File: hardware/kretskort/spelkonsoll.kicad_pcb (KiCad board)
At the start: 2 copper layers, 2 parts, among them U2 ESP32-DEVKITC-32D, U3 ILI9488

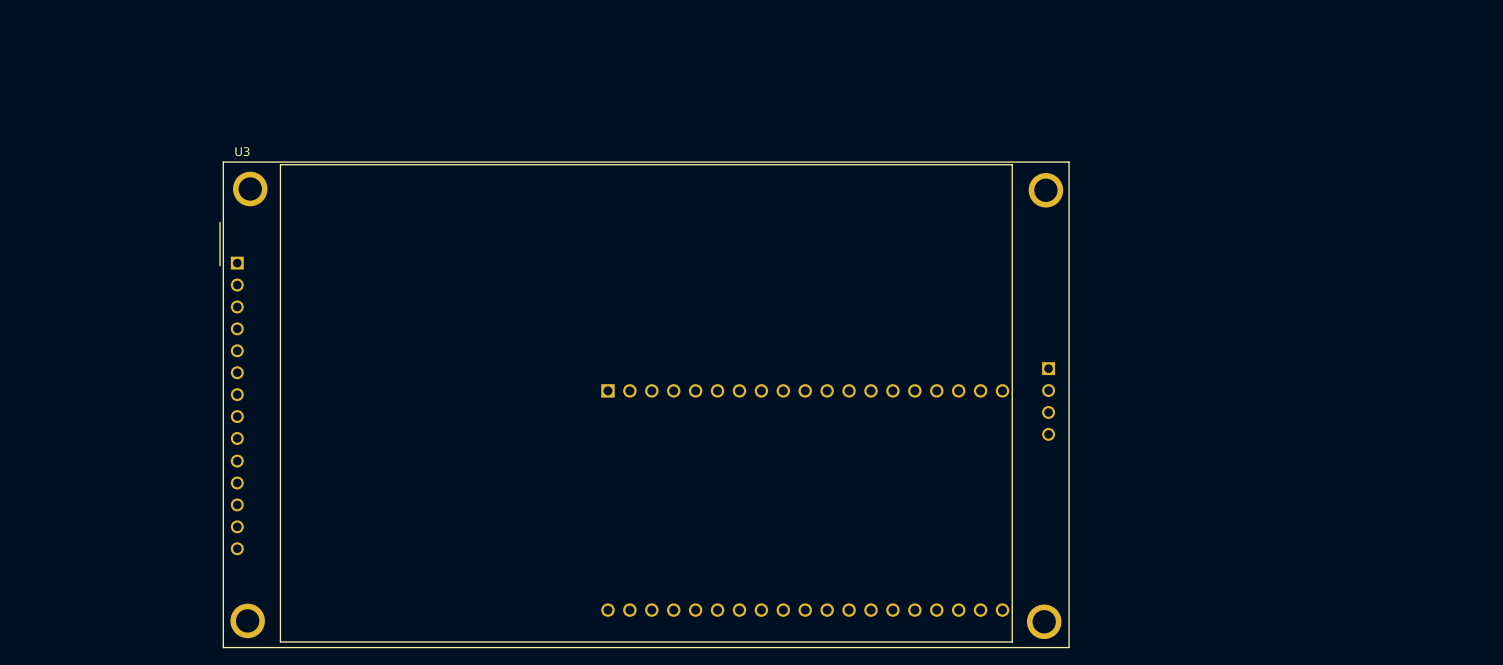
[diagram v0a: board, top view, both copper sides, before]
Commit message: more circuit board kicad files
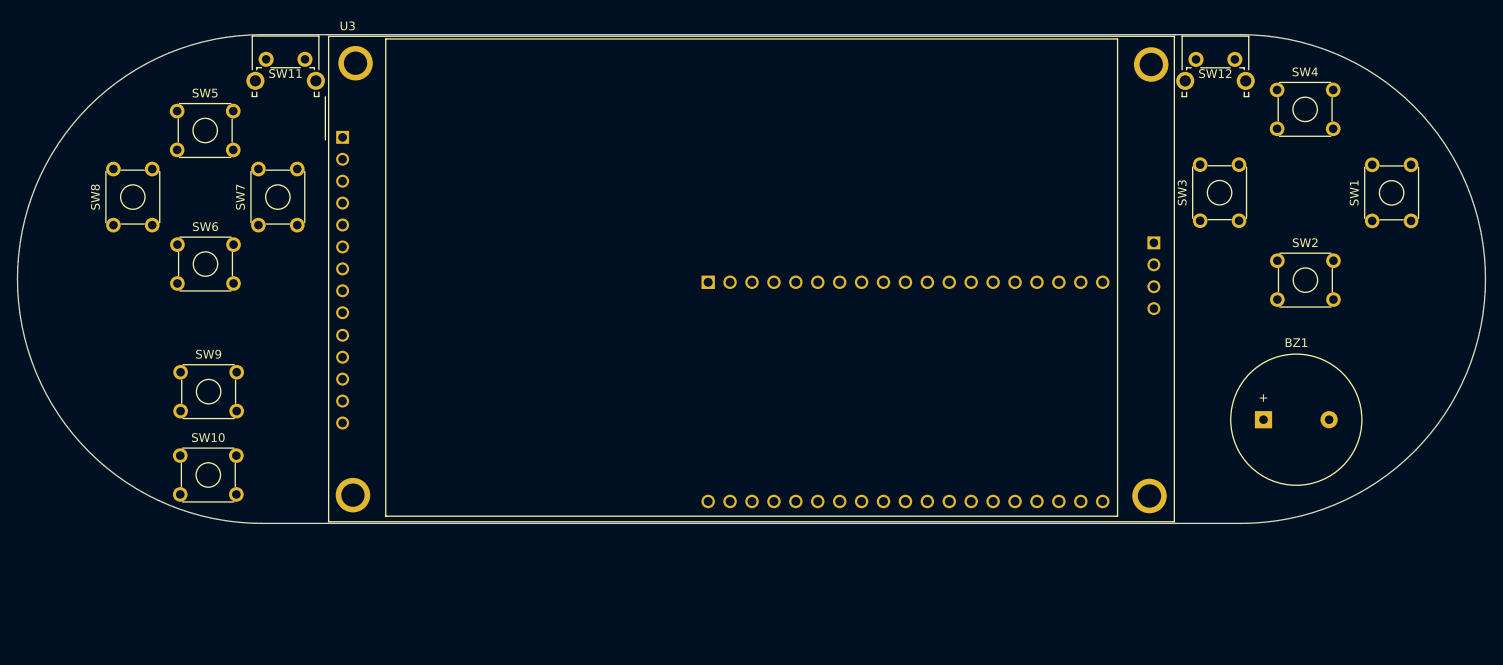
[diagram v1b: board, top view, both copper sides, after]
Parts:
- added BZ1: Buzzer, Buzzer_Beeper:Buzzer_15x7.5RM7.6, F.Cu at (204.8, 113.8)
- added SW1: SW_Push, Button_Switch_THT:SW_TH_Tactile_Omron_B3F-10xx, F.Cu at (217.4, 90.8)
- added SW10: SW_Push, Button_Switch_THT:SW_TH_Tactile_Omron_B3F-10xx, F.Cu at (79.3, 118.0)
- added SW11: SW_Push, Button_Switch_THT:SW_Tactile_SPST_Angled_PTS645Vx83-2LFS, F.Cu at (89.2, 72.1)
- added SW12: SW_Push, Button_Switch_THT:SW_Tactile_SPST_Angled_PTS645Vx83-2LFS, F.Cu at (197.0, 72.1)
- added SW2: SW_Push, Button_Switch_THT:SW_TH_Tactile_Omron_B3F-10xx, F.Cu at (206.4, 95.4)
- added SW3: SW_Push, Button_Switch_THT:SW_TH_Tactile_Omron_B3F-10xx, F.Cu at (197.5, 90.8)
- added SW4: SW_Push, Button_Switch_THT:SW_TH_Tactile_Omron_B3F-10xx, F.Cu at (206.4, 75.6)
- added SW5: SW_Push, Button_Switch_THT:SW_TH_Tactile_Omron_B3F-10xx, F.Cu at (78.9, 78.1)
- added SW6: SW_Push, Button_Switch_THT:SW_TH_Tactile_Omron_B3F-10xx, F.Cu at (78.9, 93.5)
- added SW7: SW_Push, Button_Switch_THT:SW_TH_Tactile_Omron_B3F-10xx, F.Cu at (88.3, 91.3)
- added SW8: SW_Push, Button_Switch_THT:SW_TH_Tactile_Omron_B3F-10xx, F.Cu at (71.5, 91.3)
- added SW9: SW_Push, Button_Switch_THT:SW_TH_Tactile_Omron_B3F-10xx, F.Cu at (79.3, 108.3)
- moved U3 19.0 mm to (150.2, 106.6)
- moved U2 17.1 mm to (160.2, 110.6)
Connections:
- U2 pad 10: Net-(U2-Pad10) -> BTN_SELECT
- U2 pad 11: Net-(U2-Pad11) -> BTN_DP_UP
- U2 pad 12: Net-(U2-Pad12) -> BTN_DP_DOWN
- U2 pad 13: Net-(U2-Pad13) -> BTN_DP_LEFT
- U2 pad 15: Net-(U2-Pad15) -> BTN_DP_RIGHT
- U2 pad 18: GND -> Net-(U2-Pad18)
- U2 pad 25: Net-(U2-Pad25) -> BUZZER
- U2 pad 30: Net-(U2-Pad30) -> BTN_BUMPER_L
- U2 pad 31: Net-(U2-Pad31) -> BTN_BUMPER_R
- U2 pad 5: Net-(U2-Pad5) -> BTN_A
- U2 pad 6: Net-(U2-Pad6) -> BTN_B
- U2 pad 7: Net-(U2-Pad7) -> BTN_X
- U2 pad 8: Net-(U2-Pad8) -> BTN_Y
- U2 pad 9: Net-(U2-Pad9) -> BTN_START
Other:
- board outline added: 170.1 x 56.6 mm
